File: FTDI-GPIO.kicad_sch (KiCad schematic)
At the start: 33 parts, among them J701 USB_C_Receptacle_USB2.0, U701 FT2232HL, U702 93LC56BT-I/OT, Y701 12MHz

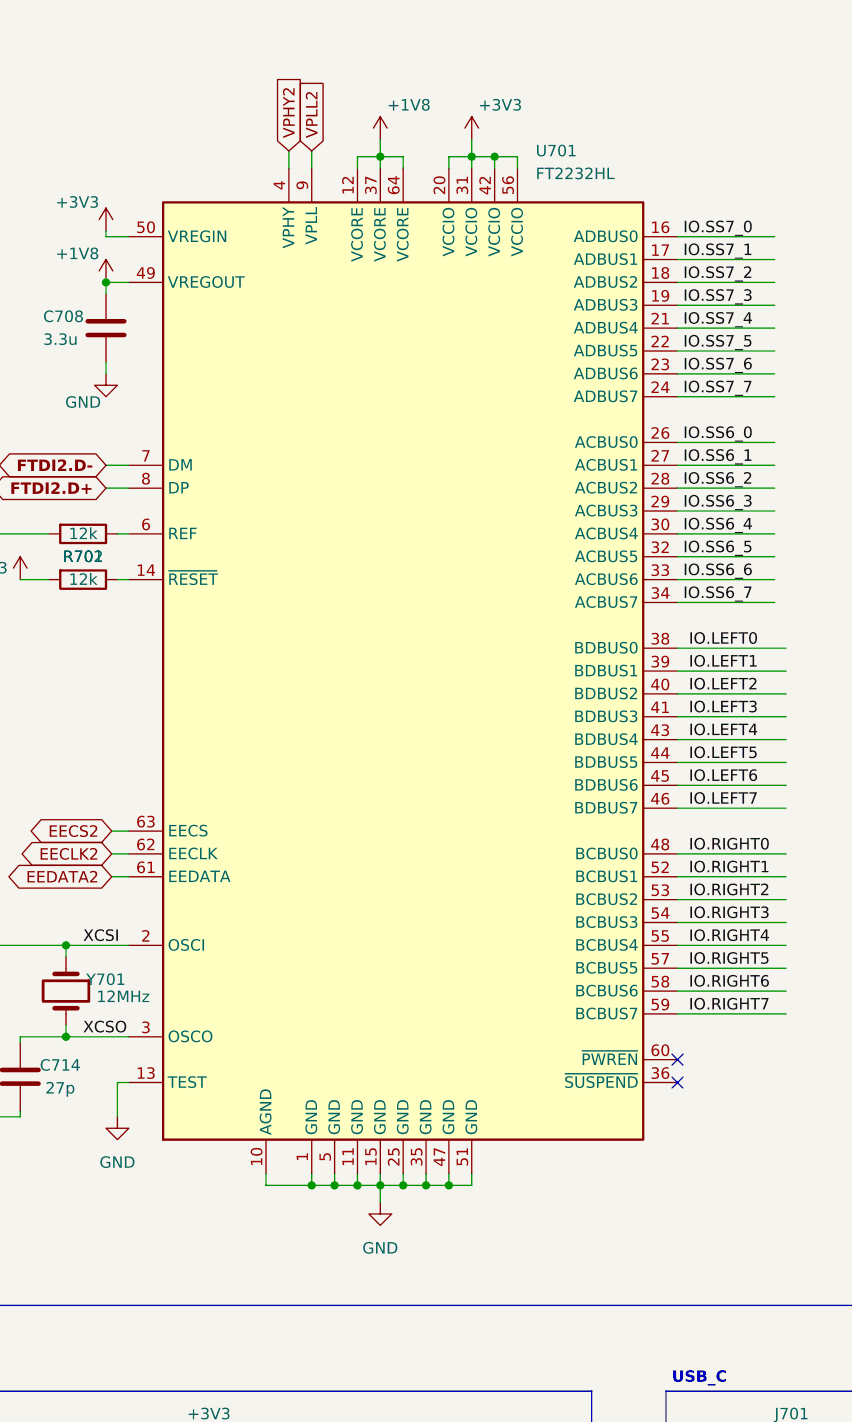
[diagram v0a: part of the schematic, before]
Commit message: Complete Design v2
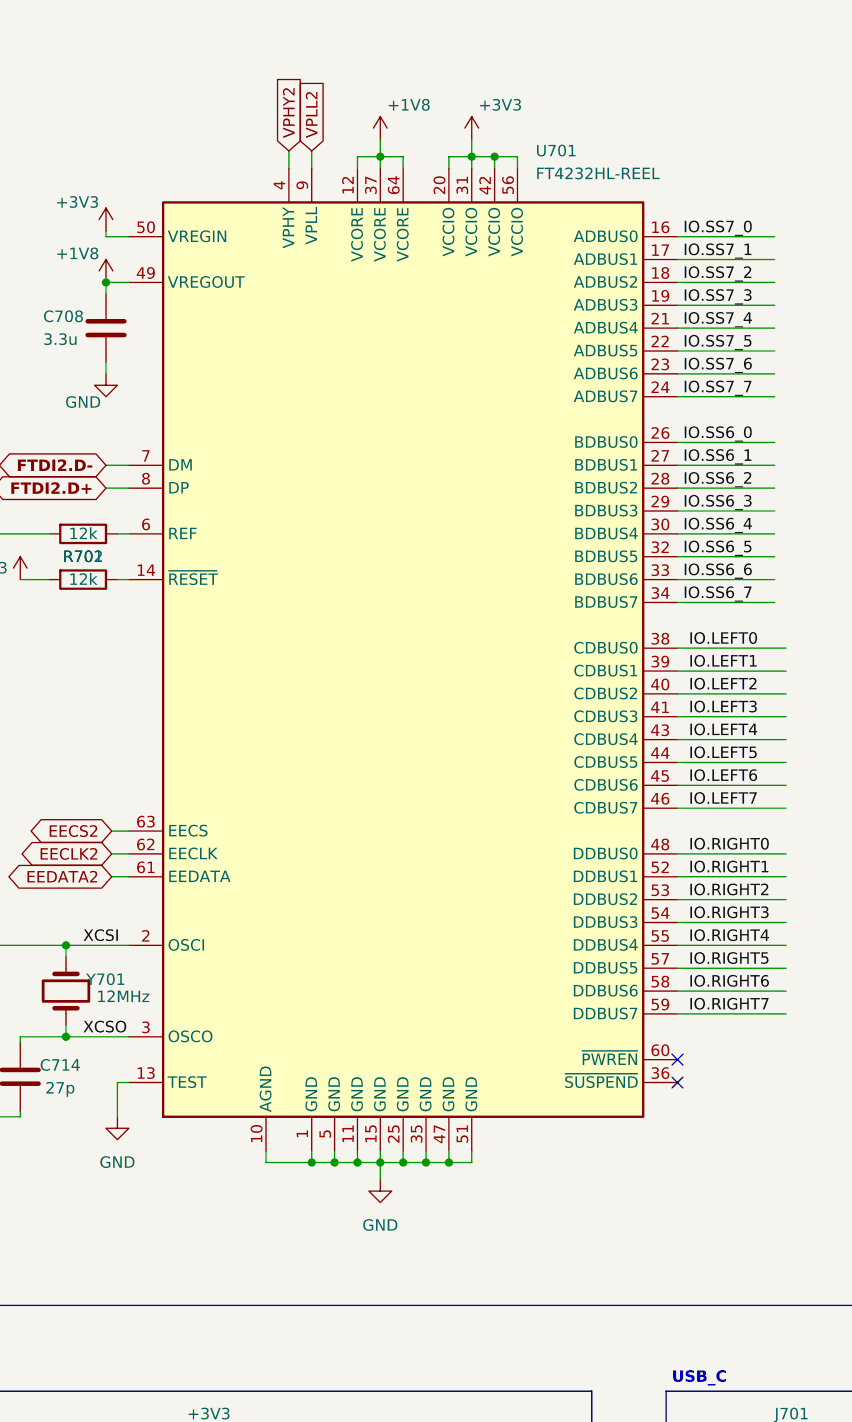
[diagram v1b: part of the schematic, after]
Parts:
- U701: value FT2232HL -> FT4232HL-REEL; symbol Interface_USB:FT2232HL -> Interface_USB:FT4232H; LCSC C27882 -> C56742; LCSC Part Number C27882 -> C56742
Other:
- moved on the sheet: U701
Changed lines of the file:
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@@
   (junction (at 80.645 187.96) (diameter 0) (color 0 0 0 0)
   )
-  (junction (at 85.09 157.48) (diameter 0) (color 0 0 0 0)
+  (junction (at 85.09 154.94) (diameter 0) (color 0 0 0 0)
   )
   (junction (at 179.705 69.215) (diameter 0) (color 0 0 0 0)
@@
   (junction (at 176.53 69.215) (diameter 0) (color 0 0 0 0)
   )
-  (junction (at 74.93 157.48) (diameter 0) (color 0 0 0 0)
+  (junction (at 74.93 154.94) (diameter 0) (color 0 0 0 0)
   )
-  (junction (at 80.01 157.48) (diameter 0) (color 0 0 0 0)
+  (junction (at 80.01 154.94) (diameter 0) (color 0 0 0 0)
   )
   (junction (at 207.01 232.41) (diameter 0) (color 0 0 0 0)
   )
-  (junction (at 77.47 157.48) (diameter 0) (color 0 0 0 0)
+  (junction (at 77.47 154.94) (diameter 0) (color 0 0 0 0)
   )
   (junction (at 210.185 44.45) (diameter 0) (color 0 0 0 0)
@@
   (junction (at 95.25 43.18) (diameter 0) (color 0 0 0 0)
   )
-  (junction (at 87.63 157.48) (diameter 0) (color 0 0 0 0)
+  (junction (at 87.63 154.94) (diameter 0) (color 0 0 0 0)
   )
-  (junction (at 90.17 157.48) (diameter 0) (color 0 0 0 0)
+  (junction (at 90.17 154.94) (diameter 0) (color 0 0 0 0)
   )
   (junction (at 173.355 34.925) (diameter 0) (color 0 0 0 0)
@@
   (junction (at 223.52 69.215) (diameter 0) (color 0 0 0 0)
   )
-  (junction (at 82.55 157.48) (diameter 0) (color 0 0 0 0)
+  (junction (at 82.55 154.94) (diameter 0) (color 0 0 0 0)
   )
   (junction (at 145.415 205.74) (diameter 0) (color 0 0 0 0)
@@
     (stroke (width 0) (type default) (color 0 0 0 0))
   )
-  (wire (pts (xy 69.85 156.21) (xy 69.85 157.48))
+  (wire (pts (xy 69.85 153.67) (xy 69.85 154.94))
     (stroke (width 0) (type default) (color 0 0 0 0))
   )
@@
     (stroke (width 0) (type default) (color 0 0 0 0))
   )
-  (wire (pts (xy 69.85 157.48) (xy 74.93 157.48))
+  (wire (pts (xy 69.85 154.94) (xy 74.93 154.94))
     (stroke (width 0) (type default) (color 0 0 0 0))
   )
@@
     (stroke (width 0) (type default) (color 0 0 0 0))
   )
-  (wire (pts (xy 90.17 157.48) (xy 92.71 157.48))
+  (wire (pts (xy 90.17 154.94) (xy 92.71 154.94))
     (stroke (width 0) (type default) (color 0 0 0 0))
   )
@@
     (stroke (width 0) (type default) (color 0 0 0 0))
   )
-  (wire (pts (xy 85.09 157.48) (xy 87.63 157.48))
+  (wire (pts (xy 85.09 154.94) (xy 87.63 154.94))
     (stroke (width 0) (type default) (color 0 0 0 0))
   )
@@
     (stroke (width 0) (type default) (color 0 0 0 0))
   )
-  (wire (pts (xy 77.47 157.48) (xy 80.01 157.48))
+  (wire (pts (xy 77.47 154.94) (xy 80.01 154.94))
     (stroke (width 0) (type default) (color 0 0 0 0))
   )
@@
     (stroke (width 0) (type default) (color 0 0 0 0))
   )
-  (wire (pts (xy 87.63 156.21) (xy 87.63 157.48))
+  (wire (pts (xy 87.63 153.67) (xy 87.63 154.94))
     (stroke (width 0) (type default) (color 0 0 0 0))
   )
@@
     (stroke (width 0) (type default) (color 0 0 0 0))
   )
-  (wire (pts (xy 90.17 156.21) (xy 90.17 157.48))
+  (wire (pts (xy 90.17 153.67) (xy 90.17 154.94))
     (stroke (width 0) (type default) (color 0 0 0 0))
   )
@@
     (stroke (width 0) (type default) (color 0 0 0 0))
   )
-  (wire (pts (xy 87.63 157.48) (xy 90.17 157.48))
+  (wire (pts (xy 87.63 154.94) (xy 90.17 154.94))
     (stroke (width 0) (type default) (color 0 0 0 0))
   )
@@
     (stroke (width 0) (type default) (color 0 0 0 0))
   )
-  (wire (pts (xy 82.55 157.48) (xy 85.09 157.48))
+  (wire (pts (xy 82.55 154.94) (xy 85.09 154.94))
     (stroke (width 0) (type default) (color 0 0 0 0))
   )
@@
     (stroke (width 0) (type default) (color 0 0 0 0))
   )
-  (wire (pts (xy 82.55 157.48) (xy 82.55 159.385))
+  (wire (pts (xy 82.55 154.94) (xy 82.55 156.845))
     (stroke (width 0) (type default) (color 0 0 0 0))
   )
@@
     (stroke (width 0) (type default) (color 0 0 0 0))
   )
-  (wire (pts (xy 82.55 156.21) (xy 82.55 157.48))
+  (wire (pts (xy 82.55 153.67) (xy 82.55 154.94))
     (stroke (width 0) (type default) (color 0 0 0 0))
   )
@@
     (stroke (width 0) (type default) (color 0 0 0 0))
   )
-  (wire (pts (xy 92.71 156.21) (xy 92.71 157.48))
+  (wire (pts (xy 92.71 153.67) (xy 92.71 154.94))
     (stroke (width 0) (type default) (color 0 0 0 0))
   )
@@
     (stroke (width 0) (type default) (color 0 0 0 0))
   )
-  (wire (pts (xy 74.93 156.21) (xy 74.93 157.48))
+  (wire (pts (xy 74.93 153.67) (xy 74.93 154.94))
     (stroke (width 0) (type default) (color 0 0 0 0))
   )
@@
     (stroke (width 0) (type default) (color 0 0 0 0))
   )
-  (wire (pts (xy 77.47 156.21) (xy 77.47 157.48))
+  (wire (pts (xy 77.47 153.67) (xy 77.47 154.94))
     (stroke (width 0) (type default) (color 0 0 0 0))
   )
@@
     (stroke (width 0) (type default) (color 0 0 0 0))
   )
-  (wire (pts (xy 74.93 157.48) (xy 77.47 157.48))
+  (wire (pts (xy 74.93 154.94) (xy 77.47 154.94))
     (stroke (width 0) (type default) (color 0 0 0 0))
   )
@@
     (stroke (width 0) (type default) (color 0 0 0 0))
   )
-  (wire (pts (xy 85.09 156.21) (xy 85.09 157.48))
+  (wire (pts (xy 85.09 153.67) (xy 85.09 154.94))
     (stroke (width 0) (type default) (color 0 0 0 0))
   )
@@
     (stroke (width 0) (type default) (color 0 0 0 0))
   )
-  (wire (pts (xy 80.01 157.48) (xy 82.55 157.48))
+  (wire (pts (xy 80.01 154.94) (xy 82.55 154.94))
     (stroke (width 0) (type default) (color 0 0 0 0))
   )
@@
     (stroke (width 0) (type default) (color 0 0 0 0))
   )
-  (wire (pts (xy 80.01 156.21) (xy 80.01 157.48))
+  (wire (pts (xy 80.01 153.67) (xy 80.01 154.94))
     (stroke (width 0) (type default) (color 0 0 0 0))
   )
@@
     (pin "1")
   )
-  (symbol (lib_id "power:GND") (at 82.55 159.385 0) (unit 1)
+  (symbol (lib_id "power:GND") (at 82.55 156.845 0) (unit 1)
     (in_bom yes) (on_board yes) (fields_autoplaced)
-    (property "Reference" "#PWR0718" (id 0) (at 82.55 165.735 0)
+    (property "Reference" "#PWR0718" (id 0) (at 82.55 163.195 0)
       (effects (font (size 1.27 1.27)) hide)
     )
-    (property "Value" "GND" (id 1) (at 82.55 164.465 0))
-    (property "Footprint" "" (id 2) (at 82.55 159.385 0)
+    (property "Value" "GND" (id 1) (at 82.55 161.925 0))
+    (property "Footprint" "" (id 2) (at 82.55 156.845 0)
       (effects (font (size 1.27 1.27)) hide)
     )
-    (property "Datasheet" "" (id 3) (at 82.55 159.385 0)
+    (property "Datasheet" "" (id 3) (at 82.55 156.845 0)
       (effects (font (size 1.27 1.27)) hide)
     )
@@
     (pin "2")
   )
-  (symbol (lib_id "Interface_USB:FT2232HL") (at 85.09 100.33 0) (unit 1)
+  (symbol (lib_id "Interface_USB:FT4232H") (at 85.09 100.33 0) (unit 1)
     (in_bom yes) (on_board yes) (fields_autoplaced)
     (property "Reference" "U701" (id 0) (at 99.8094 42.545 0)
       (effects (font (size 1.27 1.27)) (justify left))
     )
-    (property "Value" "FT2232HL" (id 1) (at 99.8094 45.085 0)
+    (property "Value" "FT4232HL-REEL" (id 1) (at 99.8094 45.085 0)
       (effects (font (size 1.27 1.27)) (justify left))
     )
@@
       (effects (font (size 1.27 1.27)) hide)
     )
-    (property "Datasheet" "https://www.ftdichip.com/Support/Documents/DataSheets/ICs/DS_FT2232H.pdf" (id 3) (at 85.09 100.33 0)
+    (property "Datasheet" "https://ftdichip.com/wp-content/uploads/2020/08/DS_FT4232H.pdf" (id 3) (at 85.09 100.33 0)
       (effects (font (size 1.27 1.27)) hide)
     )
-    (property "LCSC" "C27882" (id 4) (at 85.09 100.33 0)
+    (property "LCSC" "C56742" (id 4) (at 85.09 100.33 0)
       (effects (font (size 1.27 1.27)) hide)
     )
-    (property "LCSC Part Number" "C27882" (id 5) (at 85.09 100.33 0)
+    (property "LCSC Part Number" "C56742" (id 5) (at 85.09 100.33 0)
       (effects (font (size 1.27 1.27)) hide)
     )
